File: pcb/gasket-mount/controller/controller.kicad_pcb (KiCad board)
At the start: 2 copper layers, 26 x 28.5 mm, 39 parts, among them J1 TYPE-C-31-M-12, J2 I2C, J3 PWR, U1 USBLC6-2SC6, U2 TF31-18S-0.5SH(800), U4 RP2040, U5 AP2112K-3.3, X1 ABM8-272-T3

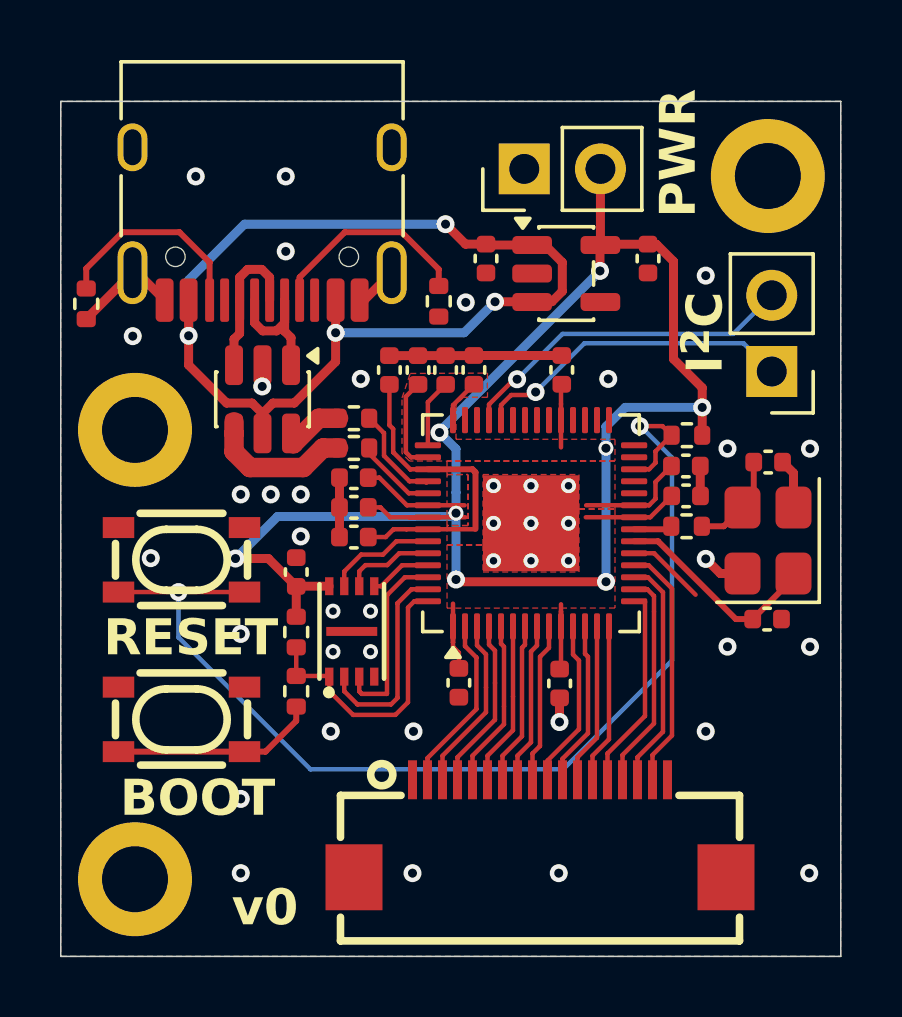
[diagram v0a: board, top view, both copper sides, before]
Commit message: rebuild #2329423
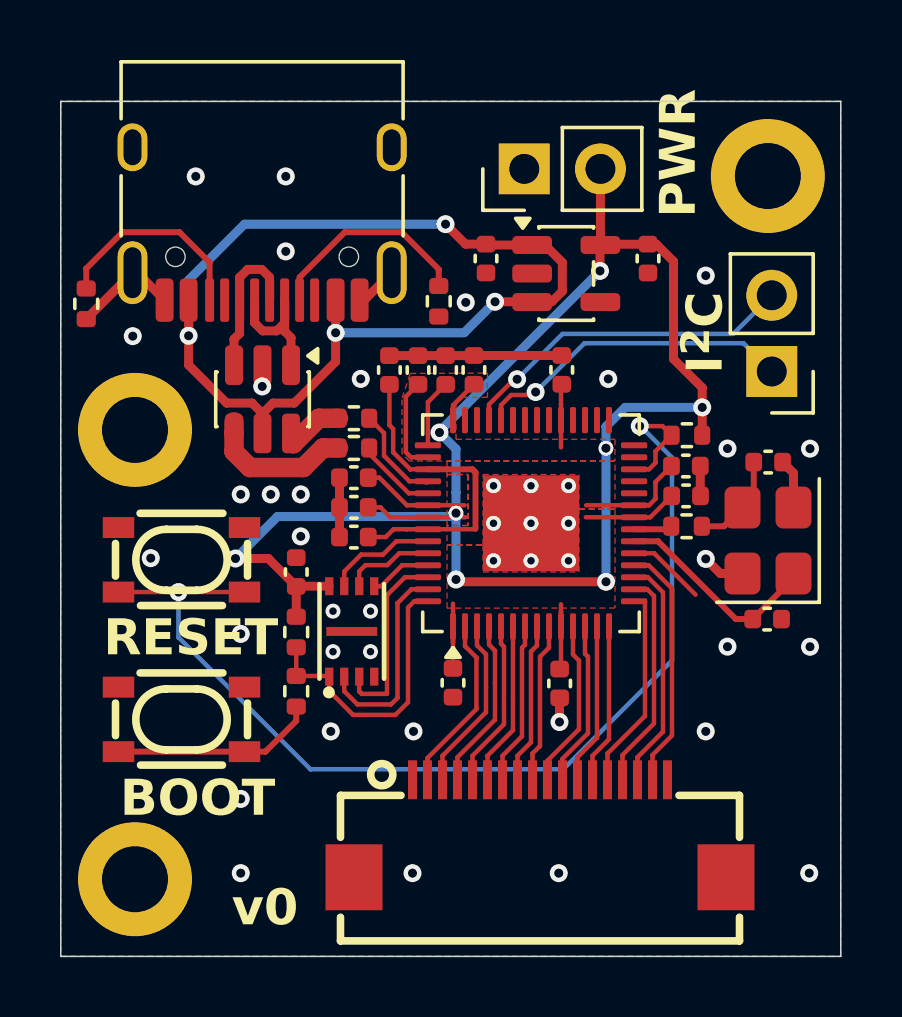
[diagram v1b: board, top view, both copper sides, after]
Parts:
- moved C9 0.20 mm to (152.3, 107.9)
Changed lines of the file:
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@@
 	(footprint "Capacitor_SMD:C_0402_1005Metric"
 		(layer "F.Cu")
-		(at 152.495837 107.935425 -90)
+		(at 152.3 107.935425 -90)
 		(descr "Capacitor SMD 0402 (1005 Metric), square (rectangular) end terminal, IPC-7351 nominal, (Body size source: IPC-SM-782 page 76, https://www.pcb-3d.com/wordpress/wp-content/uploads/ipc-sm-782a_amendment_1_and_2.pdf)")
 		(tags "capacitor")
@@
 	)
 	(segment
+		(start 152.299999 106.59281)
+		(end 152.3 107.455425)
+		(width 0.15)
+		(layer "F.Cu")
+		(net "+3V3")
+	)
+	(segment
 		(start 158.769068 93.316662)
 		(end 157.224069 93.316662)
@@
 	)
 	(segment
-		(start 152.495837 106.931163)
-		(end 152.299999 106.735327)
-		(width 0.15)
-		(layer "F.Cu")
-		(net "+3V3")
-	)
-	(segment
 		(start 147.075 105.732811)
 		(end 147.075 104.72281)
 		(width 0.3)
-		(layer "F.Cu")
-		(net "+3V3")
-	)
-	(segment
-		(start 152.495837 106.931163)
-		(end 152.495837 107.455425)
-		(width 0.15)
 		(layer "F.Cu")
 		(net "+3V3")
@@
 		(layer "F.Cu")
 		(net "+3V3")
-	)
-	(segment
-		(start 152.299999 106.735327)
-		(end 152.299999 106.59281)
-		(width 0.15)
-		(layer "F.Cu")
-		(net "+3V3")
